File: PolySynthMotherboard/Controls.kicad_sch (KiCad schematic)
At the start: 92 parts, among them SW601 ENV1_B, SW602 ENV2_B, SW603 LFO1_B, SW604 LFO2_B, SW605 LFO3_B, SW606 MIX1_B, SW607 MIX2_B, SW608 MENU_B, SW609 FF_B, SW610 HP_B, SW611 HP_B, U204 ILI9341, U501 MCP23S17_SS

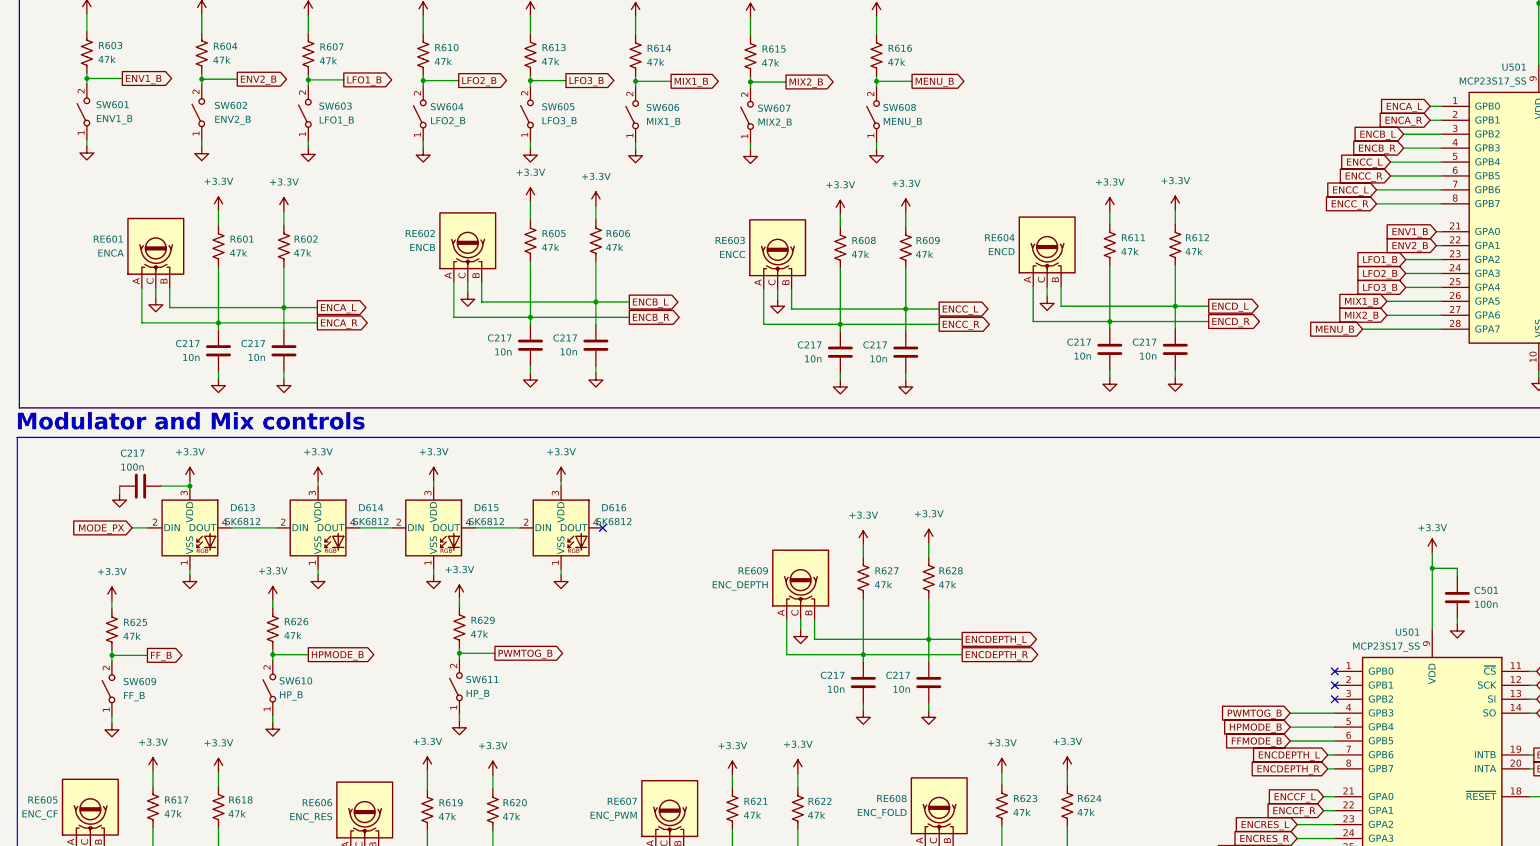
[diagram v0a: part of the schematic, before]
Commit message: board layout
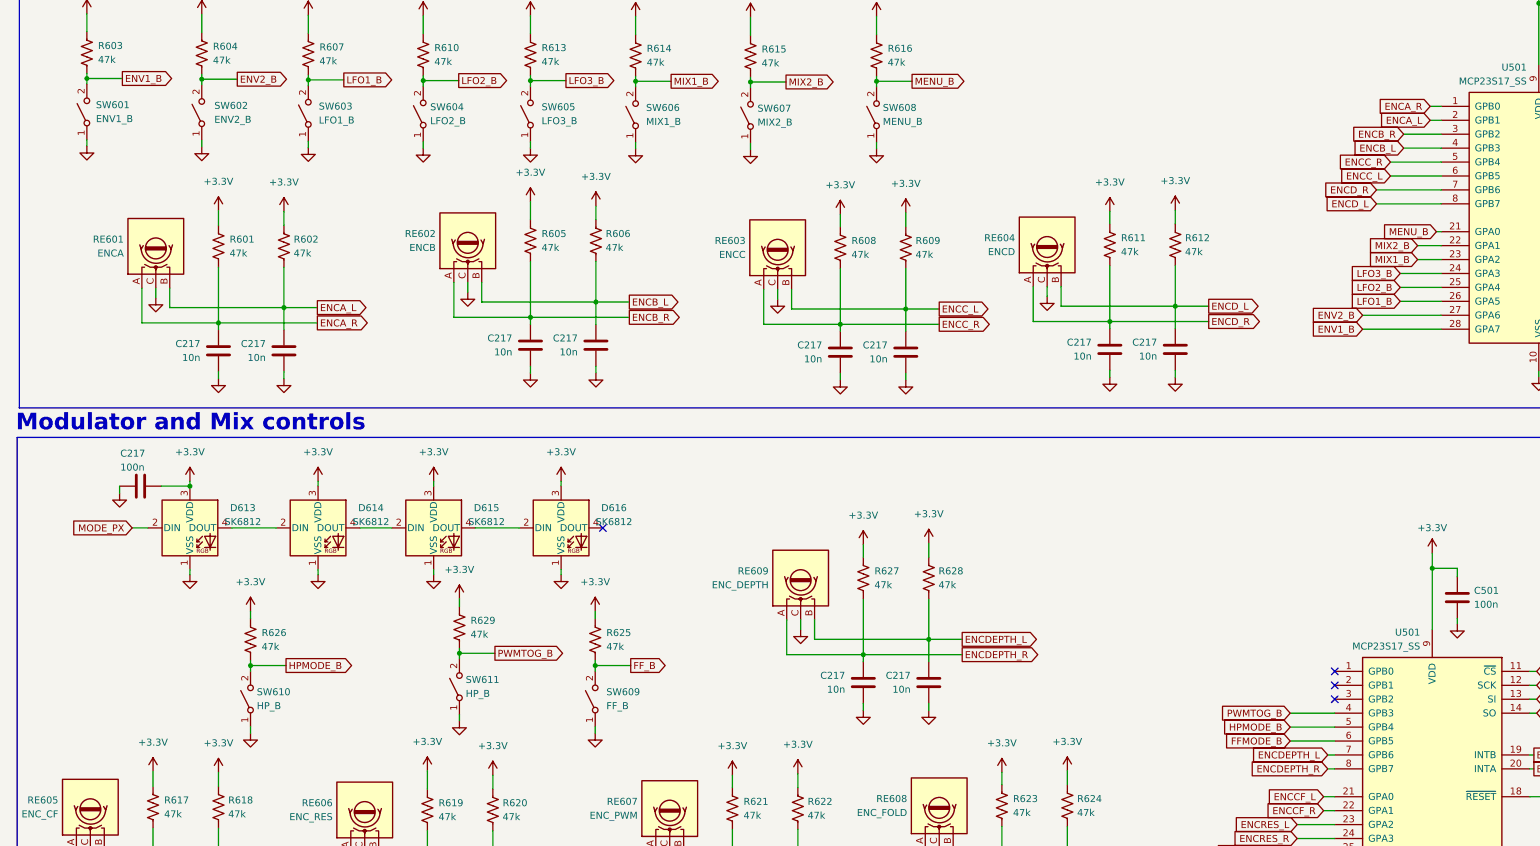
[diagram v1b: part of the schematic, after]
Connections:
- net ENCA_L: now also U501.2 (GPB1); no longer U501.1 (GPB0)
- net ENCA_R: now also U501.1 (GPB0); no longer U501.2 (GPB1)
- net ENCB_L: now also U501.4 (GPB3); no longer U501.3 (GPB2)
- net ENCB_R: now also U501.3 (GPB2); no longer U501.4 (GPB3)
- net ENCC_L: now also U501.6 (GPB5); no longer U501.5 (GPB4), U501.7 (GPB6)
- net ENCC_R: now also U501.5 (GPB4); no longer U501.6 (GPB5), U501.8 (GPB7)
- net ENCD_L: now also U501.8 (GPB7)
- net ENCD_R: now also U501.7 (GPB6)
- net ENV1_B: now also U501.28 (GPA7); no longer U501.21 (GPA0)
- net ENV2_B: now also U501.27 (GPA6); no longer U501.22 (GPA1)
- net LFO1_B: now also U501.26 (GPA5); no longer U501.23 (GPA2)
- net LFO2_B: now also U501.25 (GPA4); no longer U501.24 (GPA3)
- net LFO3_B: now also U501.24 (GPA3); no longer U501.25 (GPA4)
- net MENU_B: now also U501.21 (GPA0); no longer U501.28 (GPA7)
- net MIX1_B: now also U501.23 (GPA2); no longer U501.26 (GPA5)
- net MIX2_B: now also U501.22 (GPA1); no longer U501.27 (GPA6)
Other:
- moved on the sheet: R625, R626, SW609, SW610
